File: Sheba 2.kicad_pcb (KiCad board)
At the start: 2 copper layers, 85.7 x 54 mm, 68 parts, among them J1 Conn_01x03_Pin, J2 Conn_01x03_Pin, J3 Conn_01x03_Pin, J4 Conn_01x03_Pin, J5 Jack-DC, J6 GPIO, J7 Conn_01x06_Pin, J8 Conn_01x02_Pin, SW1 SW_SPDT, U1 AP62150Z6, U2 STM32H503CBTx, U3 MIC5504-3.3YM5

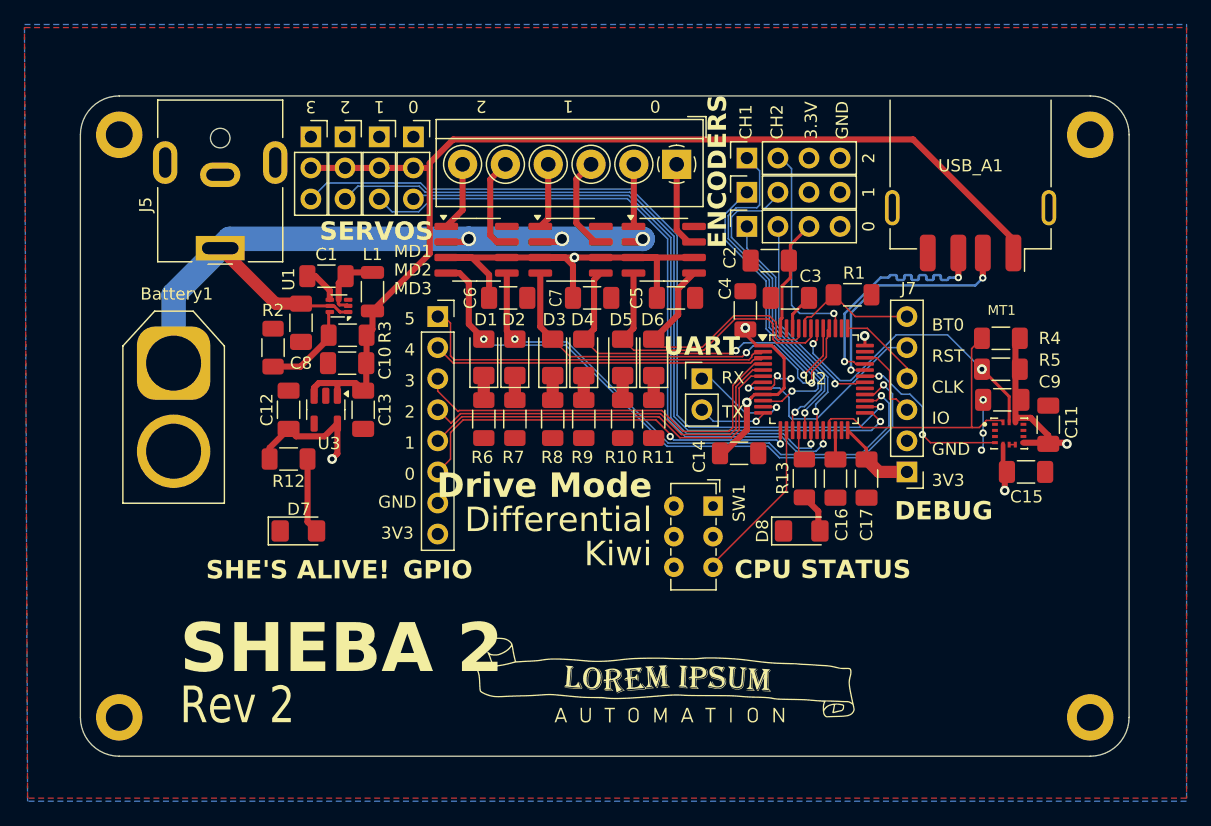
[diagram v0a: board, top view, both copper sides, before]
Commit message: Rev 2 ordered!
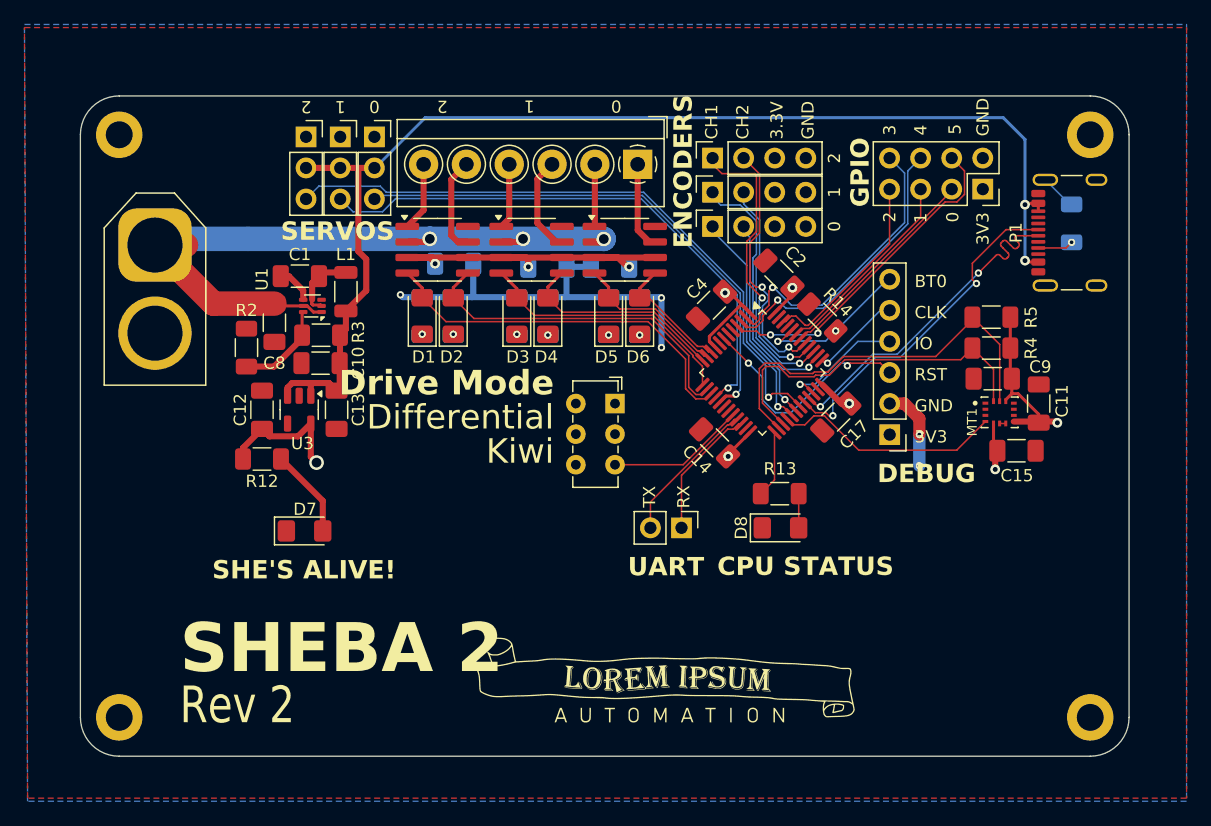
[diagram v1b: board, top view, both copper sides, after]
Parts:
- removed C16, C3: C2.2uF, Capacitor_SMD:C_1206_3216Metric_Pad1.33x1.80mm_HandSolder
- removed J1: Conn_01x03_Pin, Connector_PinSocket_2.54mm:PinSocket_1x03_P2.54mm_Vertical
- removed J5: Jack-DC, Connector_BarrelJack:BarrelJack_CUI_PJ-063AH_Horizontal
- removed J6: GPIO, Connector_PinSocket_2.54mm:PinSocket_1x08_P2.54mm_Vertical
- removed U2: STM32H503CBTx, Package_QFP:LQFP-48_7x7mm_P0.5mm
- removed USB_A1: USB_A, Connector_USB:USB_A_Receptacle_GCT_USB1046
- added J9: Conn_02x04_Top_Bottom, Connector_PinSocket_2.54mm:PinSocket_2x04_P2.54mm_Vertical, F.Cu at (127.1, 37.6)
- added P1: USB_C_Plug_USB2.0, Connector_USB:USB_C_Receptacle_GCT_USB4105-xx-A_16P_TopMnt_Horizontal, F.Cu at (135.3, 41.1)
- added R14: R10k, Resistor_SMD:R_1206_3216Metric_Pad1.30x1.75mm_HandSolder, F.Cu at (114.0, 48.1)
- added U4: STM32F072CBTx, Package_QFP:LQFP-48_7x7mm_P0.5mm, F.Cu at (109.1, 52.6)
- C5, C6, C7, R10, R11, R6, R7, R8, R9: moved to B.Cu
- R1: value R10k -> 5.11K; moved to B.Cu
- moved R1 18.8 mm to (134.4, 40.4), turned to -90 degrees
- moved J8 12.3 mm to (102.5, 65.3), turned to -90 degrees
- moved SW1 11.6 mm to (97.0, 55.1)
- moved R6 9.81 mm to (81.3, 48.0), turned to 90 degrees
- moved R7 9.81 mm to (83.8, 48.0), turned to 90 degrees
- moved Battery1 9.77 mm to (59.4, 42.2)
- moved R9 8.91 mm to (91.6, 48.0), turned to 90 degrees
- moved R8 8.91 mm to (89.0, 48.0), turned to 90 degrees
- moved R10 8.50 mm to (96.5, 48.0), turned to 90 degrees
- moved R11 8.50 mm to (99.1, 48.0), turned to 90 degrees
- moved D1 6.06 mm to (81.3, 48.0)
- moved D2 6.06 mm to (83.8, 48.0)
- moved C5 5.96 mm to (96.6, 43.9), turned to 180 degrees
- moved C17 5.62 mm to (115.1, 56.2), turned to -135 degrees
- moved C6 5.22 mm to (83.9, 43.7)
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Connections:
- net I2C1_SCL renamed I2C2_SCL
- net I2C1_SDA renamed I2C2_SDA
- C17 pad 1: GND -> +3V3
- C17 pad 2: +3V3 -> GND
- C2 pad 1: +3V3 -> GND
- C2 pad 2: GND -> +3V3
- J2 pad 3: SERVO_2 -> SERVO2
- J3 pad 3: SERVO_1 -> SERVO1
- J4 pad 3: SERVO_0 -> SERVO0
- J7 pad 3: SYS_SWDIO -> NRST
- J7 pad 4: SYS_SWCLK -> SYS_SWDIO
- J7 pad 5: NRST -> SYS_SWCLK
- J8 pad 1: USART1_RX -> USART3_RX
- J8 pad 2: USART1_TX -> USART3_TX
- R1 pad 1: BOOT0 -> GND
- R1 pad 2: GND -> Net-(P1-CC)
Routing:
- net SERVO_3: track 66.0 -> 0.00 mm, vias 1 -> 0
- net SERVO_2: track 62.4 -> 0.00 mm, vias 1 -> 0
- net SERVO_1: track 55.8 -> 0.00 mm, vias 1 -> 0
- net SERVO2: track 0.00 -> 52.4 mm, vias 0 -> 1
- net SERVO_0: track 50.9 -> 0.00 mm, vias 1 -> 0
- net SERVO1: track 0.00 -> 46.2 mm, vias 0 -> 1
- net SERVO0: track 0.00 -> 42.9 mm, vias 0 -> 1
- net GND: track 7.76 -> 43.1 mm
- net GPIO_0: track 33.1 -> 0.00 mm, vias 2 -> 0
- net GPIO_3: track 32.5 -> 0.00 mm
- net GPIO_1: track 32.3 -> 0.00 mm
- net GPIO_2: track 32.3 -> 0.00 mm
- net GPIO_5: track 29.5 -> 0.00 mm
- net USB_D-: track 0.00 -> 28.1 mm, vias 0 -> 2
- net USB_D+: track 0.00 -> 28.0 mm, vias 0 -> 2
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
